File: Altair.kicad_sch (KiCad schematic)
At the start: 2 parts, among them J1 Battery, U1 nice_nano

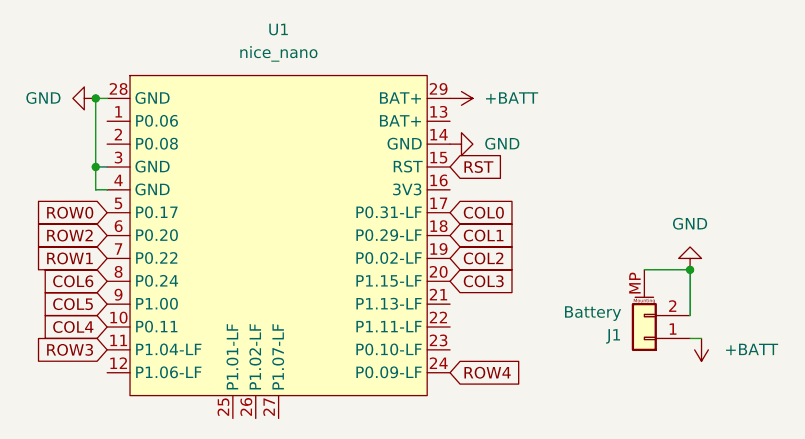
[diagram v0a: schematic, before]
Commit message: Done for 1 side PCB
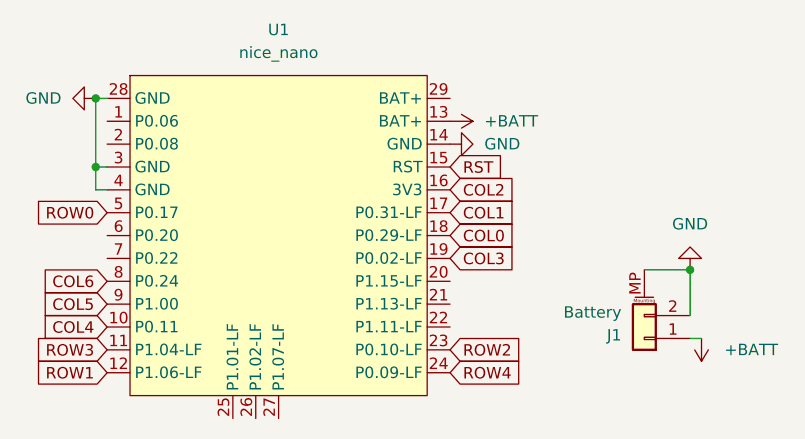
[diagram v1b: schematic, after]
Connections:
- net +BATT: now also U1.13 (BAT+); no longer U1.29 (BAT+)
- net COL0: now also U1.18 (P0.29-LF); no longer U1.17 (P0.31-LF)
- net COL1: now also U1.17 (P0.31-LF); no longer U1.18 (P0.29-LF)
- net COL2: now also U1.16 (3V3); no longer U1.19 (P0.02-LF)
- net COL3: now also U1.19 (P0.02-LF); no longer U1.20 (P1.15-LF)
- net ROW1: now also U1.12 (P1.06-LF); no longer U1.7 (P0.22)
- net ROW2: now also U1.23 (P0.10-LF); no longer U1.6 (P0.20)
